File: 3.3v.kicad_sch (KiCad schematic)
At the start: 12 parts, among them J4 Conn_01x04_Pin, J5 Conn_01x04_Pin, U4 LM2596S-3.3

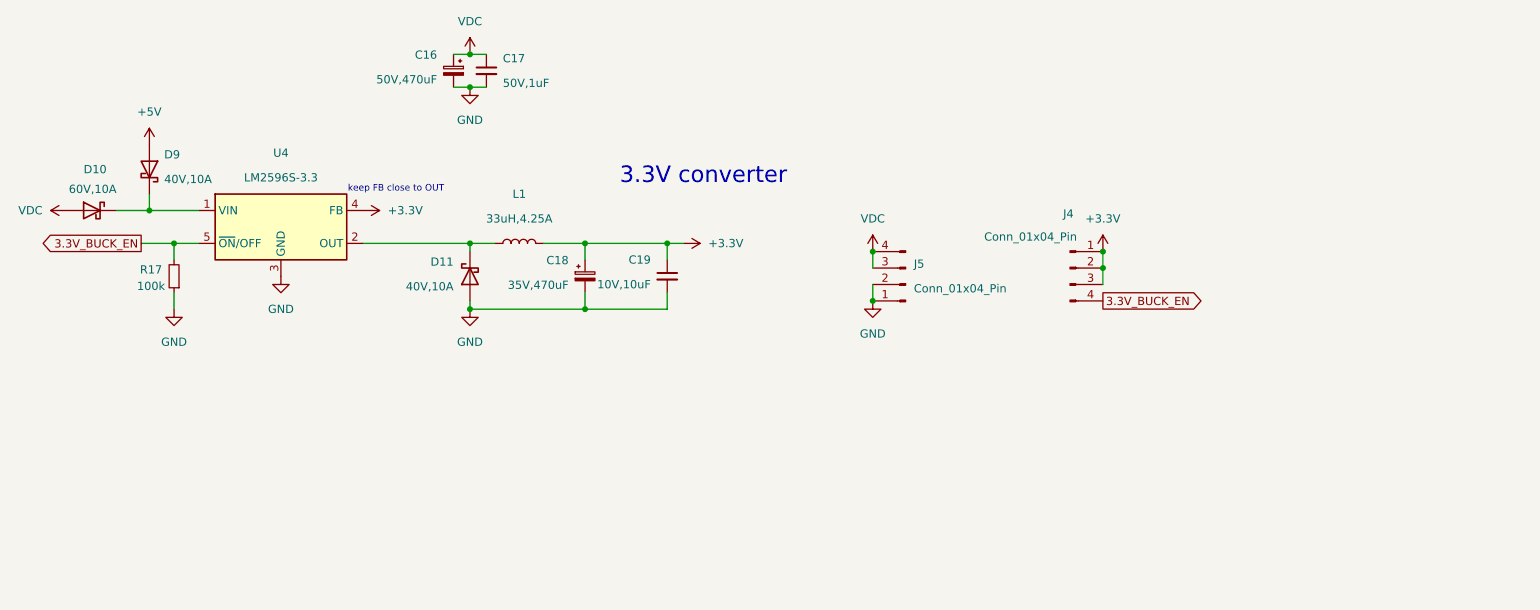
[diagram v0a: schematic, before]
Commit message: finished schematic yay!! now onto pcb routing :fire:
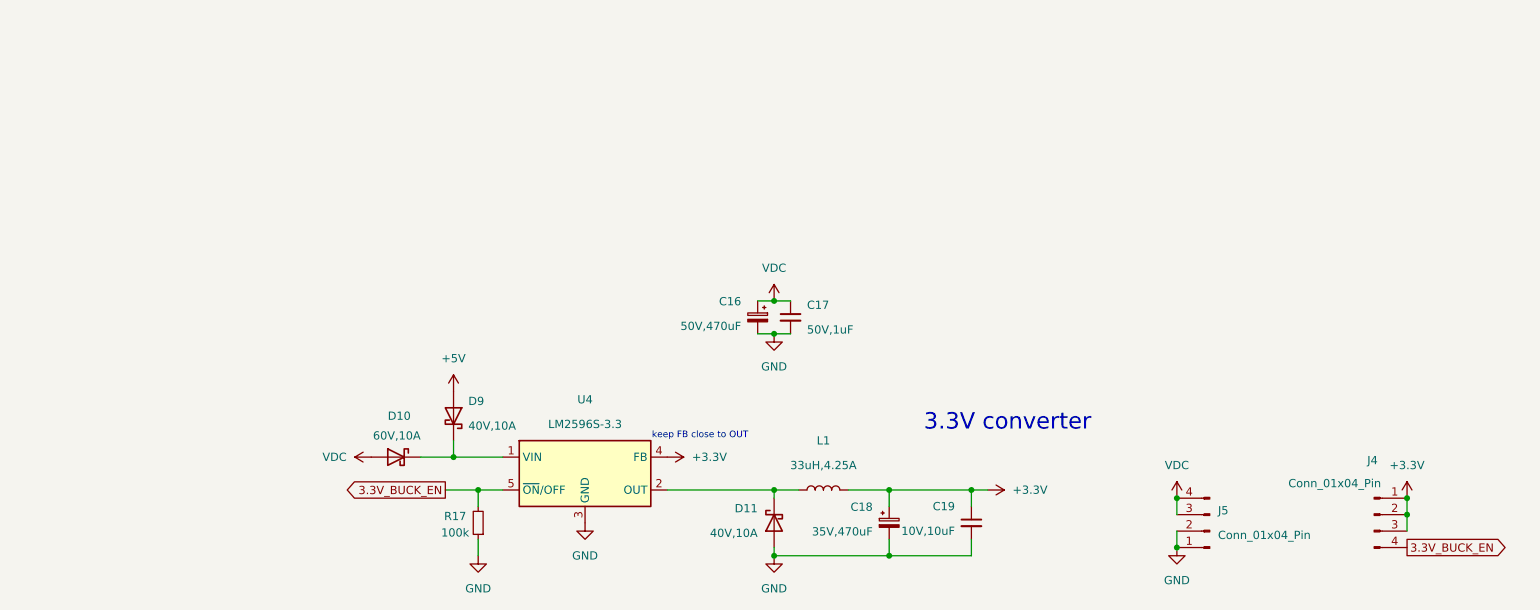
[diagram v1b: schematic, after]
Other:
- moved on the sheet: C16, C17, C18, C19, D10, D11, D9, J4, J5, L1, R17, U4
